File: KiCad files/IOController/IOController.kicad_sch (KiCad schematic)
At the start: 12 parts, among them J1 AVR-ISP-6, J2 Conn_01x01, J3 Conn_01x01, J4 Conn_01x01, J5 Conn_01x01, Q1 IRF3205, U1 ATtiny85-20P, U3 LP2985-1.8

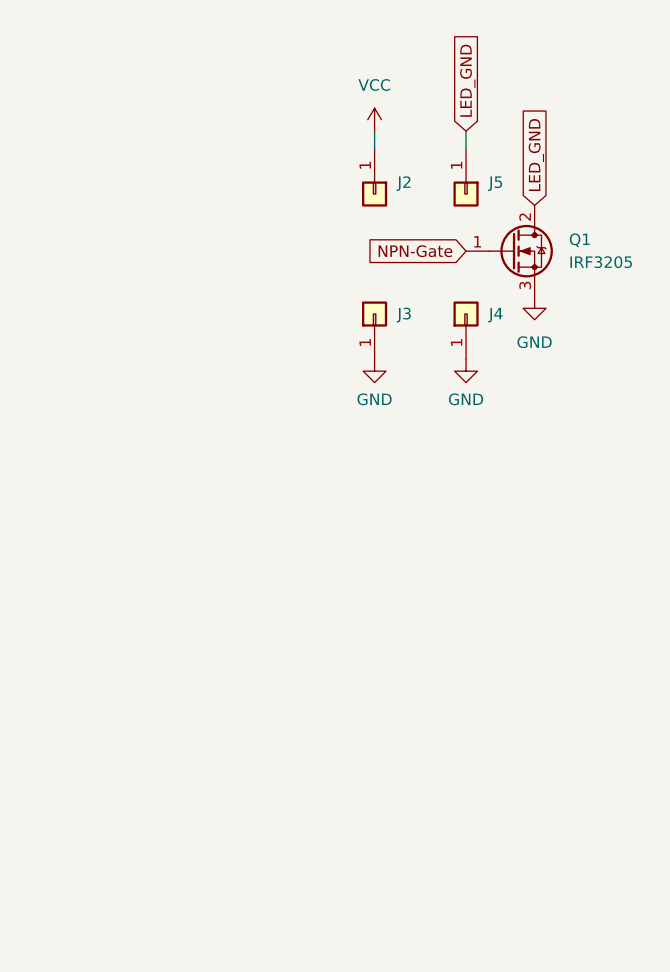
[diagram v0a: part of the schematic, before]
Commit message: added some parts to controller board for now.
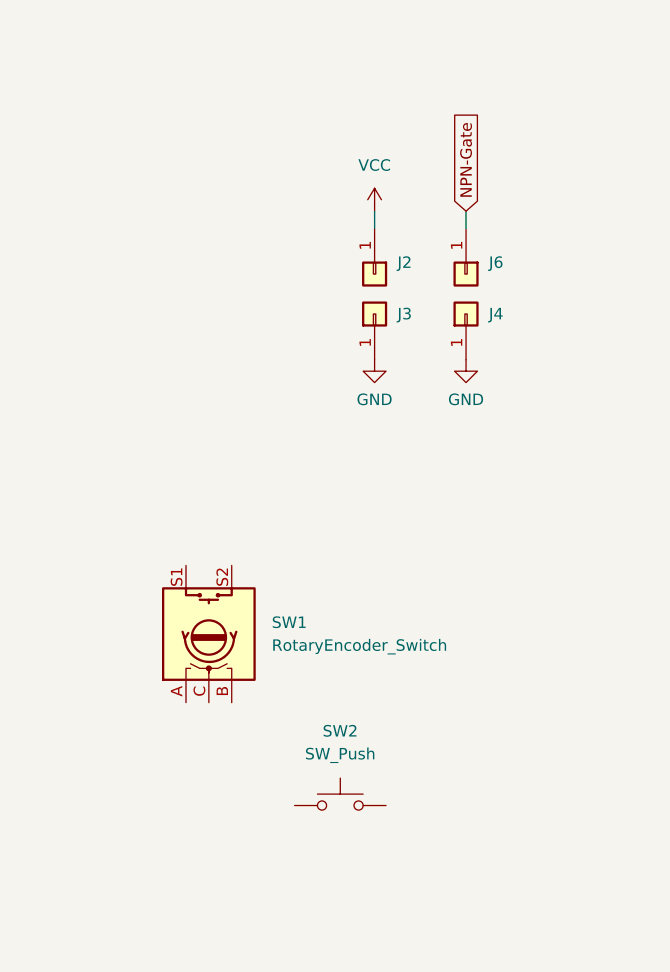
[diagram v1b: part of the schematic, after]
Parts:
- removed J5: Conn_01x01, Connector_Wire:SolderWire-2.5sqmm_1x01_D2.4mm_OD3.6mm, symbol Connector_Generic:Conn_01x01
- removed Q1: IRF3205, Package_TO_SOT_THT:TO-220-3_Vertical, symbol Transistor_FET:IRF3205
- added J6: Conn_01x01, Connector_Wire:SolderWire-2.5sqmm_1x01_D2.4mm_OD3.6mm, symbol Connector_Generic:Conn_01x01
- added SW1: RotaryEncoder_Switch, Rotary_Encoder:RotaryEncoder_Bourns_Horizontal_PEC09-2xxxF-Nxxxx, symbol Device:RotaryEncoder_Switch
- added SW2: SW_Push, symbol Switch:SW_Push
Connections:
- net NPN-Gate: now also J6.1 (Pin_1)
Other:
- moved on the sheet: J2
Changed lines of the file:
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@@
+    (stroke (width 0) (type default))
+  )
+  (wire (pts (xy 146.05 34.29) (xy 146.05 32.385))
     (stroke (width 0) (type default))
   )
@@
     (stroke (width 0) (type default))
   )
-  (wire (pts (xy 135.89 25.4) (xy 135.89 23.495))
+  (wire (pts (xy 135.89 34.29) (xy 135.89 32.385))
     (stroke (width 0) (type default))
   )
@@
     (stroke (width 0) (type default))
   )
-  (wire (pts (xy 146.05 25.4) (xy 146.05 23.495))
-    (stroke (width 0) (type default))
-  )
   (wire (pts (xy 76.2 76.835) (xy 65.405 76.835))
     (stroke (width 0) (type default))
@@
     (stroke (width 0) (type default))
   )
-  (global_label "NPN-Gate" (shape input) (at 146.05 36.83 180) (fields_autoplaced)
-    (effects (font (size 1.27 1.27)) (justify right))
-    (property "Intersheetrefs" "${INTERSHEET_REFS}" (at 133.3281 36.83 0)
-      (effects (font (size 1.27 1.27)) (justify right) hide)
-    )
-  )
-  (global_label "LED_GND" (shape input) (at 153.67 31.75 90) (fields_autoplaced)
+  (global_label "NPN-Gate" (shape input) (at 146.05 32.385 90) (fields_autoplaced)
     (effects (font (size 1.27 1.27)) (justify left))
-    (property "Intersheetrefs" "${INTERSHEET_REFS}" (at 153.67 20.4796 90)
+    (property "Intersheetrefs" "${INTERSHEET_REFS}" (at 146.05 19.6631 90)
       (effects (font (size 1.27 1.27)) (justify left) hide)
     )
@@
     )
   )
-  (global_label "LED_GND" (shape input) (at 146.05 23.495 90) (fields_autoplaced)
-    (effects (font (size 1.27 1.27)) (justify left))
-    (property "Intersheetrefs" "${INTERSHEET_REFS}" (at 146.05 12.2246 90)
+  (symbol (lib_id "Connector_Generic:Conn_01x01") (at 135.89 39.37 270) (unit 1)
+    (in_bom yes) (on_board yes) (dnp no)
+    (property "Reference" "J2" (at 138.43 38.1 90)
+      (effects (font (size 1.27 1.27)) (justify left))
+    )
+    (property "Value" "Conn_01x01" (at 138.43 40.64 90)
       (effects (font (size 1.27 1.27)) (justify left) hide)
     )
-  )
-  (symbol (lib_id "Connector_Generic:Conn_01x01") (at 135.89 30.48 270) (unit 1)
-    (in_bom yes) (on_board yes) (dnp no) (fields_autoplaced)
-    (property "Reference" "J2" (at 138.43 29.21 90)
-      (effects (font (size 1.27 1.27)) (justify left))
-    )
-    (property "Value" "Conn_01x01" (at 138.43 31.75 90)
-      (effects (font (size 1.27 1.27)) (justify left) hide)
-    )
-    (property "Footprint" "Connector_Wire:SolderWire-2.5sqmm_1x01_D2.4mm_OD3.6mm" (at 135.89 30.48 0)
-      (effects (font (size 1.27 1.27)) hide)
-    )
-    (property "Datasheet" "~" (at 135.89 30.48 0)
+    (property "Footprint" "Connector_Wire:SolderWire-2.5sqmm_1x01_D2.4mm_OD3.6mm" (at 135.89 39.37 0)
+      (effects (font (size 1.27 1.27)) hide)
+    )
+    (property "Datasheet" "~" (at 135.89 39.37 0)
       (effects (font (size 1.27 1.27)) hide)
     )
@@
     )
   )
+  (symbol (lib_id "Switch:SW_Push") (at 132.08 98.425 0) (unit 1)
+    (in_bom yes) (on_board yes) (dnp no) (fields_autoplaced)
+    (property "Reference" "SW2" (at 132.08 90.17 0)
+      (effects (font (size 1.27 1.27)))
+    )
+    (property "Value" "SW_Push" (at 132.08 92.71 0)
+      (effects (font (size 1.27 1.27)))
+    )
+    (property "Footprint" "" (at 132.08 93.345 0)
+      (effects (font (size 1.27 1.27)) hide)
+    )
+    (property "Datasheet" "~" (at 132.08 93.345 0)
+      (effects (font (size 1.27 1.27)) hide)
+    )
+    (pin "2")
+    (pin "1")
+    (instances
+      (project "IOController"
+        (path "/f1c719f6-f1ad-4e81-8891-bde8a483290d"
+          (reference "SW2") (unit 1)
+        )
+      )
+    )
+  )
   (symbol (lib_id "power:GND") (at 50.165 86.995 0) (unit 1)
     (in_bom yes) (on_board yes) (dnp no) (fields_autoplaced)
@@
         (path "/f1c719f6-f1ad-4e81-8891-bde8a483290d"
           (reference "#PWR02") (unit 1)
-        )
-      )
-    )
-  )
-  (symbol (lib_id "Connector_Generic:Conn_01x01") (at 146.05 30.48 270) (unit 1)
-    (in_bom yes) (on_board yes) (dnp no) (fields_autoplaced)
-    (property "Reference" "J5" (at 148.59 29.21 90)
-      (effects (font (size 1.27 1.27)) (justify left))
-    )
-    (property "Value" "Conn_01x01" (at 148.59 31.75 90)
-      (effects (font (size 1.27 1.27)) (justify left) hide)
-    )
-    (property "Footprint" "Connector_Wire:SolderWire-2.5sqmm_1x01_D2.4mm_OD3.6mm" (at 146.05 30.48 0)
-      (effects (font (size 1.27 1.27)) hide)
-    )
-    (property "Datasheet" "~" (at 146.05 30.48 0)
-      (effects (font (size 1.27 1.27)) hide)
-    )
-    (pin "1")
-    (instances
-      (project "IOController"
-        (path "/f1c719f6-f1ad-4e81-8891-bde8a483290d"
-          (reference "J5") (unit 1)
         )
       )
@@
     )
   )
-  (symbol (lib_id "power:VCC") (at 135.89 23.495 0) (unit 1)
-    (in_bom yes) (on_board yes) (dnp no) (fields_autoplaced)
-    (property "Reference" "#PWR08" (at 135.89 27.305 0)
-      (effects (font (size 1.27 1.27)) hide)
-    )
-    (property "Value" "VCC" (at 135.89 18.415 0)
-      (effects (font (size 1.27 1.27)))
-    )
-    (property "Footprint" "" (at 135.89 23.495 0)
-      (effects (font (size 1.27 1.27)) hide)
-    )
-    (property "Datasheet" "" (at 135.89 23.495 0)
+  (symbol (lib_id "power:VCC") (at 135.89 32.385 0) (unit 1)
+    (in_bom yes) (on_board yes) (dnp no) (fields_autoplaced)
+    (property "Reference" "#PWR08" (at 135.89 36.195 0)
+      (effects (font (size 1.27 1.27)) hide)
+    )
+    (property "Value" "VCC" (at 135.89 27.305 0)
+      (effects (font (size 1.27 1.27)))
+    )
+    (property "Footprint" "" (at 135.89 32.385 0)
+      (effects (font (size 1.27 1.27)) hide)
+    )
+    (property "Datasheet" "" (at 135.89 32.385 0)
       (effects (font (size 1.27 1.27)) hide)
     )
@@
     )
   )
-  (symbol (lib_id "Transistor_FET:IRF3205") (at 151.13 36.83 0) (unit 1)
-    (in_bom yes) (on_board yes) (dnp no) (fields_autoplaced)
-    (property "Reference" "Q1" (at 157.48 35.56 0)
+  (symbol (lib_id "Connector_Generic:Conn_01x01") (at 146.05 39.37 270) (unit 1)
+    (in_bom yes) (on_board yes) (dnp no)
+    (property "Reference" "J6" (at 148.59 38.1 90)
       (effects (font (size 1.27 1.27)) (justify left))
     )
-    (property "Value" "IRF3205" (at 157.48 38.1 0)
-      (effects (font (size 1.27 1.27)) (justify left))
-    )
-    (property "Footprint" "Package_TO_SOT_THT:TO-220-3_Vertical" (at 156.21 38.735 0)
-      (effects (font (size 1.27 1.27) italic) (justify left) hide)
-    )
-    (property "Datasheet" "http://www.irf.com/product-info/datasheets/data/irf3205.pdf" (at 156.21 40.64 0)
+    (property "Value" "Conn_01x01" (at 148.59 40.64 90)
       (effects (font (size 1.27 1.27)) (justify left) hide)
     )
-    (pin "2")
-    (pin "1")
-    (pin "3")
-    (instances
-      (project "IOController"
-        (path "/f1c719f6-f1ad-4e81-8891-bde8a483290d"
-          (reference "Q1") (unit 1)
+    (property "Footprint" "Connector_Wire:SolderWire-2.5sqmm_1x01_D2.4mm_OD3.6mm" (at 146.05 39.37 0)
+      (effects (font (size 1.27 1.27)) hide)
+    )
+    (property "Datasheet" "~" (at 146.05 39.37 0)
+      (effects (font (size 1.27 1.27)) hide)
+    )
+    (pin "1")
+    (instances
+      (project "IOController"
+        (path "/f1c719f6-f1ad-4e81-8891-bde8a483290d"
+          (reference "J6") (unit 1)
         )
       )
@@
     )
   )
+  (symbol (lib_id "Device:RotaryEncoder_Switch") (at 117.475 79.375 90) (unit 1)
+    (in_bom yes) (on_board yes) (dnp no) (fields_autoplaced)
+    (property "Reference" "SW1" (at 124.46 78.105 90)
+      (effects (font (size 1.27 1.27)) (justify right))
+    )
+    (property "Value" "RotaryEncoder_Switch" (at 124.46 80.645 90)
+      (effects (font (size 1.27 1.27)) (justify right))
+    )
+    (property "Footprint" "Rotary_Encoder:RotaryEncoder_Bourns_Horizontal_PEC09-2xxxF-Nxxxx" (at 113.411 83.185 0)
+      (effects (font (size 1.27 1.27)) hide)
+    )
+    (property "Datasheet" "~" (at 110.871 79.375 0)
+      (effects (font (size 1.27 1.27)) hide)
+    )
+    (pin "S2")
+    (pin "B")
+    (pin "S1")
+    (pin "A")
+    (pin "C")
+    (instances
+      (project "IOController"
+        (path "/f1c719f6-f1ad-4e81-8891-bde8a483290d"
+          (reference "SW1") (unit 1)
+        )
+      )
+    )
+  )
   (symbol (lib_id "power:VDD") (at 50.165 56.515 0) (unit 1)
     (in_bom yes) (on_board yes) (dnp no) (fields_autoplaced)
@@
         )
       )
-    )
-  )
-  (symbol (lib_id "power:GND") (at 153.67 41.91 0) (unit 1)
-    (in_bom yes) (on_board yes) (dnp no) (fields_autoplaced)
-    (property "Reference" "#PWR011" (at 153.67 48.26 0)
-      (effects (font (size 1.27 1.27)) hide)
-    )
-    (property "Value" "GND" (at 153.67 46.99 0)
-      (effects (font (size 1.27 1.27)))
-    )
-    (property "Footprint" "" (at 153.67 41.91 0)
-      (effects (font (size 1.27 1.27)) hide)
-    )
-    (property "Datasheet" "" (at 153.67 41.91 0)
-      (effects (font (size 1.27 1.27)) hide)
-    )
-    (pin "1")
-    (instances
-      (project "IOController"
-        (path "/f1c719f6-f1ad-4e81-8891-bde8a483290d"
-          (reference "#PWR011") (unit 1)
-        )
-      )
